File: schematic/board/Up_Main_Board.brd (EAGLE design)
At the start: 79.9 x 73.5 mm, 20 parts

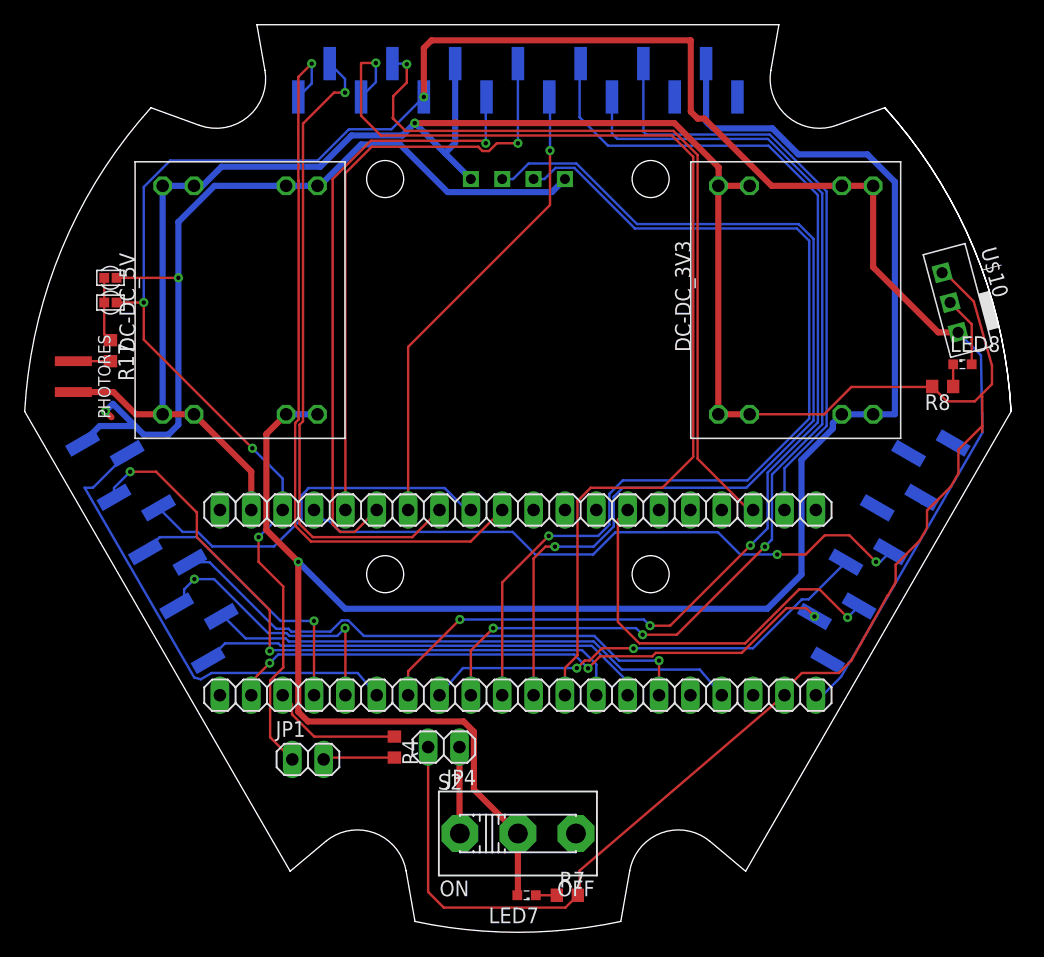
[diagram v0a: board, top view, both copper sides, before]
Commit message: ПЕРЕДЕЛАЙ ПАЛТЫ
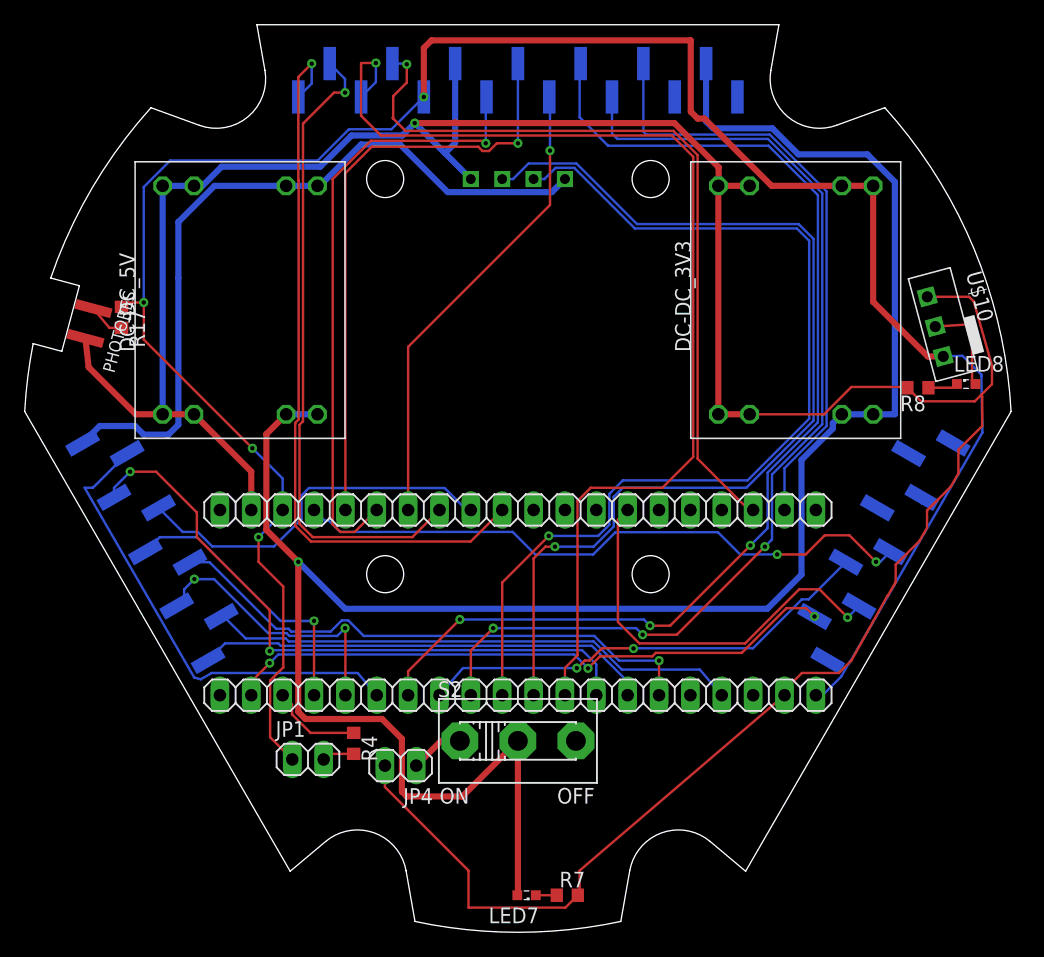
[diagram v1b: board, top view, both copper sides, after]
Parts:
- removed 3V3, 5V: (no value), NEON-BLADE-2023:VIAS-CONNECT
- R17: value 191k/2k -> 2k
- moved S2 7.50 mm to (50.0, 25.5)
- moved PHOTORES 4.49 mm to (15.3, 59.3), turned to 75 degrees
- moved JP4 3.81 mm to (40.5, 23.5)
- moved R4 3.31 mm to (36.7, 25.3)
- moved R17 2.85 mm to (17.9, 59.8)
- moved U$10 2.29 mm to (83.8, 59.0)
- moved R8 2.00 mm to (82.4, 54.1)
- moved LED8 1.63 mm to (86.3, 54.4)
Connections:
- removed net N$13: 3V3.2, 5V.1, R17.1
- net 3V3: now also R17.1; no longer 3V3.1
- net 5V: no longer 5V.2
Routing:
- net 5V: track 70.5 -> 61.4 mm, vias 2 -> 0
- net V_BAT: track 161.0 -> 168.8 mm
- net N$13: track 5.26 -> 0.00 mm
- net LED: track 10.9 -> 7.48 mm
- net N$37: track 5.79 -> 2.62 mm
- net N$1: track 7.01 -> 4.36 mm
- net STATE: track 5.74 -> 7.92 mm
- net N$10: track 1.80 -> 2.42 mm
- net GND: track 239.8 -> 240.4 mm
- net 3V3: track 181.2 -> 181.7 mm
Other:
- outline, holes or cut-outs redrawn

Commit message: исправил верхнюю плату
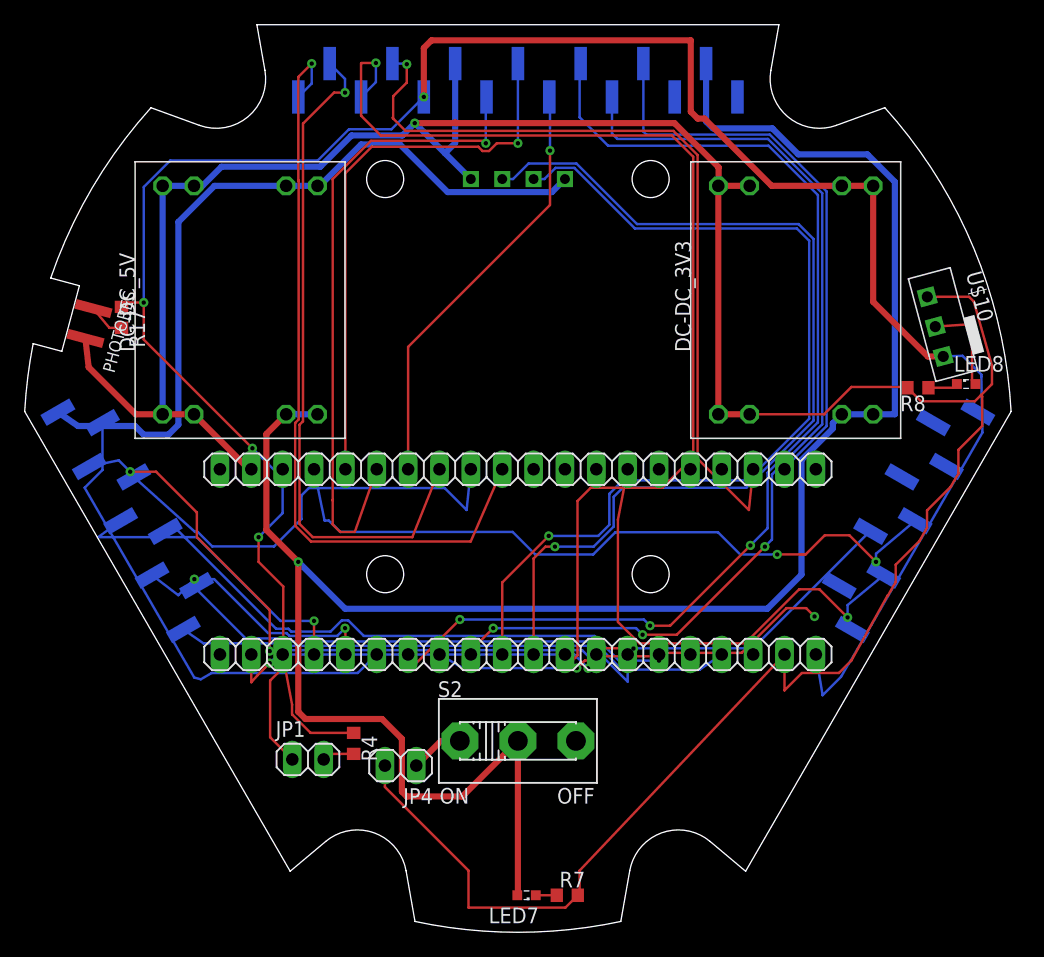
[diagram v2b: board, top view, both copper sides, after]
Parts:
- moved U$2 3.30 mm to (50.0, 40.0)
- moved U$6 3.20 mm to (81.0, 44.0)
- moved U$7 3.20 mm to (19.0, 44.0)
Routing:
- net 4MOSI: track 32.8 -> 39.3 mm
- net CS_TDC: track 51.5 -> 57.9 mm
- net SDIO_CMD: track 30.7 -> 36.8 mm
- net 3V3: track 181.7 -> 186.0 mm
- net GPS_TX: track 80.5 -> 77.2 mm
- net GPS_RX: track 82.8 -> 79.5 mm
- net CS_LSM: track 50.1 -> 46.8 mm
- net CS_NRF: track 49.5 -> 46.2 mm
- net 5SCK: track 38.4 -> 35.1 mm
- net 5MISO: track 83.9 -> 80.6 mm
- net LED: track 7.48 -> 10.5 mm
- net CS_LIS: track 62.8 -> 65.8 mm
- net SCL: track 36.9 -> 39.8 mm
- net CE_NRF: track 50.4 -> 53.3 mm
- net 1MOSI: track 52.5 -> 55.3 mm
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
